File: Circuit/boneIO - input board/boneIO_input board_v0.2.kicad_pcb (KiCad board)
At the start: 2 copper layers, 256 x 74 mm, 213 parts, among them J1 Screw_Terminal_01x08, J10 BeagleBone_Black_Header, J11 BeagleBone_Black_Header, J12 Conn_02x04_Odd_Even, J13 Screw_Terminal_01x04, J2 Screw_Terminal_01x08, J3 Screw_Terminal_01x08, J4 Screw_Terminal_01x08, J5 Screw_Terminal_01x08, J6 Screw_Terminal_01x08, J7 Screw_Terminal_01x08, J8 Screw_Terminal_01x08, J9 Screw_Terminal_01x08, SW1 SW_Push, U1 EL357N-G, U10 EL357N-G, U11 EL357N-G, U12 EL357N-G, U13 EL357N-G, U14 EL357N-G, U15 EL357N-G, U16 EL357N-G, U17 EL357N-G, U18 EL357N-G, U19 EL357N-G, U2 EL357N-G, U20 EL357N-G, U21 EL357N-G, U22 EL357N-G, U23 EL357N-G, U24 EL357N-G, U25 EL357N-G, U26 EL357N-G, U27 EL357N-G, U28 RS485, U29 EL357N-G, U3 EL357N-G, U30 EL357N-G, U31 EL357N-G, U32 EL357N-G, U33 DS1307Z+, U34 EL357N-G, U35 EL357N-G, U36 EL357N-G, U37 EL357N-G, U38 EL357N-G, U39 EL357N-G, U4 EL357N-G, U40 EL357N-G, U41 EL357N-G, U42 EL357N-G, U43 EL357N-G, U44 EL357N-G, U45 EL357N-G, U46 P82B96, U47 EL357N-G, U48 EL357N-G, U49 EL357N-G, U5 EL357N-G, U50 EL357N-G, U51 EL357N-G, U52 EL357N-G, U53 EL357N-G, U54 EL357N-G, U55 EL357N-G, U56 EL357N-G, U6 EL357N-G, U7 EL357N-G, U8 EL357N-G, U9 LM2596S-ADJ, Y1 32,788 MHz

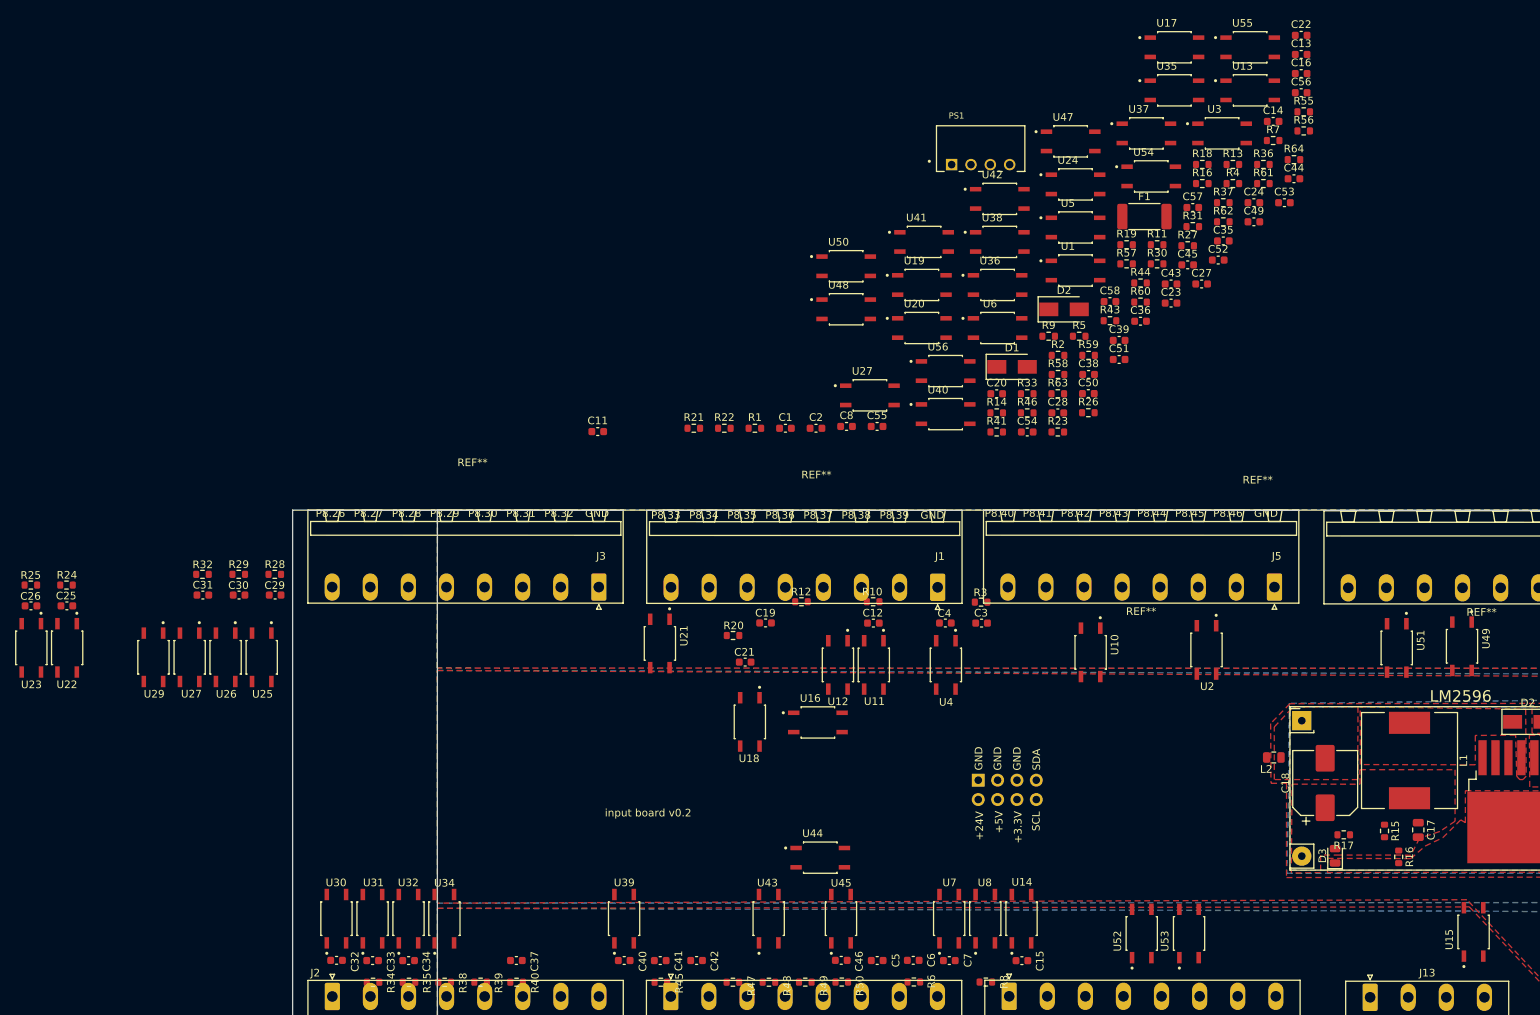
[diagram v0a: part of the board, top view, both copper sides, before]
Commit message: Revert "Zmiana Nazwy płytki"
This reverts commit 4cfb8962ad837d49dd7d8c96a90ff7a4eda2ea33.
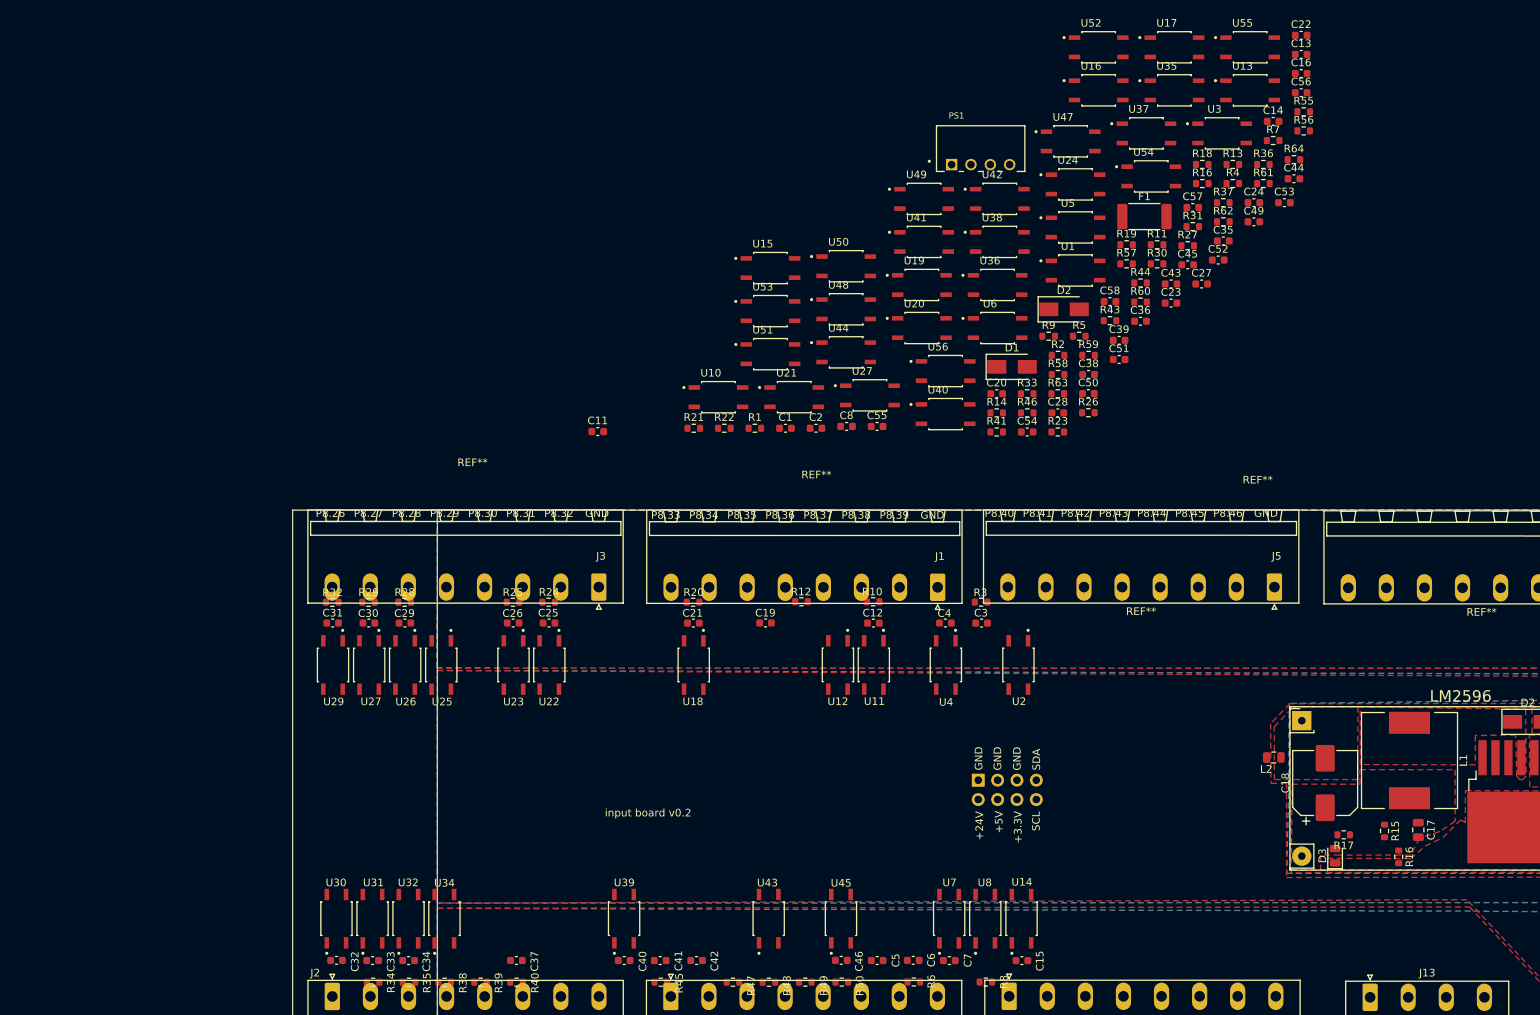
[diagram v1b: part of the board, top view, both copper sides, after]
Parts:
- moved U15 126.9 mm to (75.2, 22.1), turned to 0 degrees
- moved U52 116.5 mm to (118.3, -6.89), turned to 0 degrees
- moved U53 98.5 mm to (75.2, 27.7), turned to 0 degrees
- moved U49 91.8 mm to (95.4, 13.0), turned to 0 degrees
- moved U51 90.8 mm to (75.2, 33.4), turned to 0 degrees
- moved U16 90.8 mm to (118.3, -1.25)
- moved U44 66.4 mm to (85.1, 33.1)
- moved R24 63.3 mm to (46.1, 66.0)
- moved R25 63.3 mm to (41.4, 66.0)
- moved C25 63.3 mm to (46.1, 68.7)
- moved C26 63.3 mm to (41.4, 68.7)
- moved U23 63.3 mm to (41.5, 74.2)
- moved U22 63.3 mm to (46.2, 74.2)
- moved U10 59.2 mm to (68.4, 39.0), turned to 0 degrees
- moved U21 36.8 mm to (78.3, 39.0), turned to 0 degrees
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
